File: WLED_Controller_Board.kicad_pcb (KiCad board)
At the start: 2 copper layers, 58.2 x 43.4 mm, 21 parts, among them IC1 SN74HCT125D, J1 Barrel_Jack, J2 FTDI Programmer, J3 WLED (VCC, DI, CI, GND), J4 DHT11 / DHT22, SW1 Reset, SW2 Prog, U1 ESP-12E, U2 AMS1117-3.3

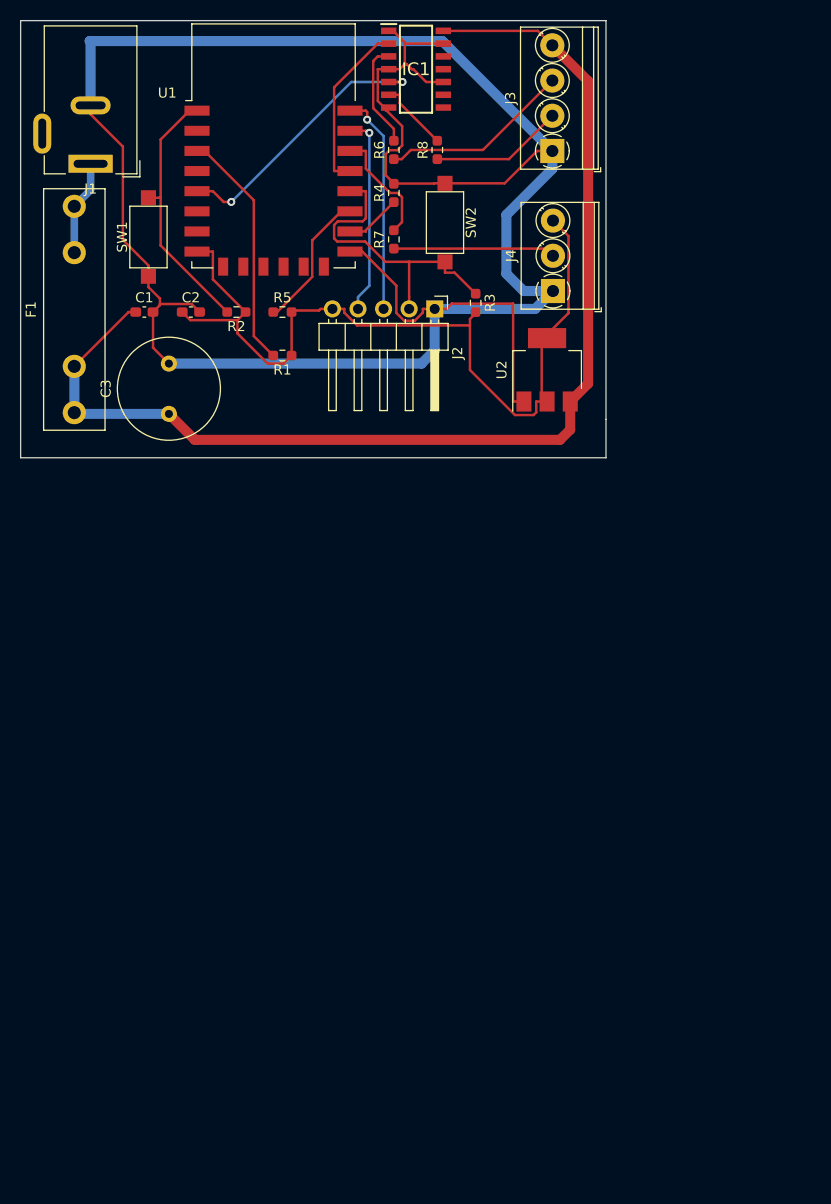
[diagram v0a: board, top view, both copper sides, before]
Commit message: Add files via upload
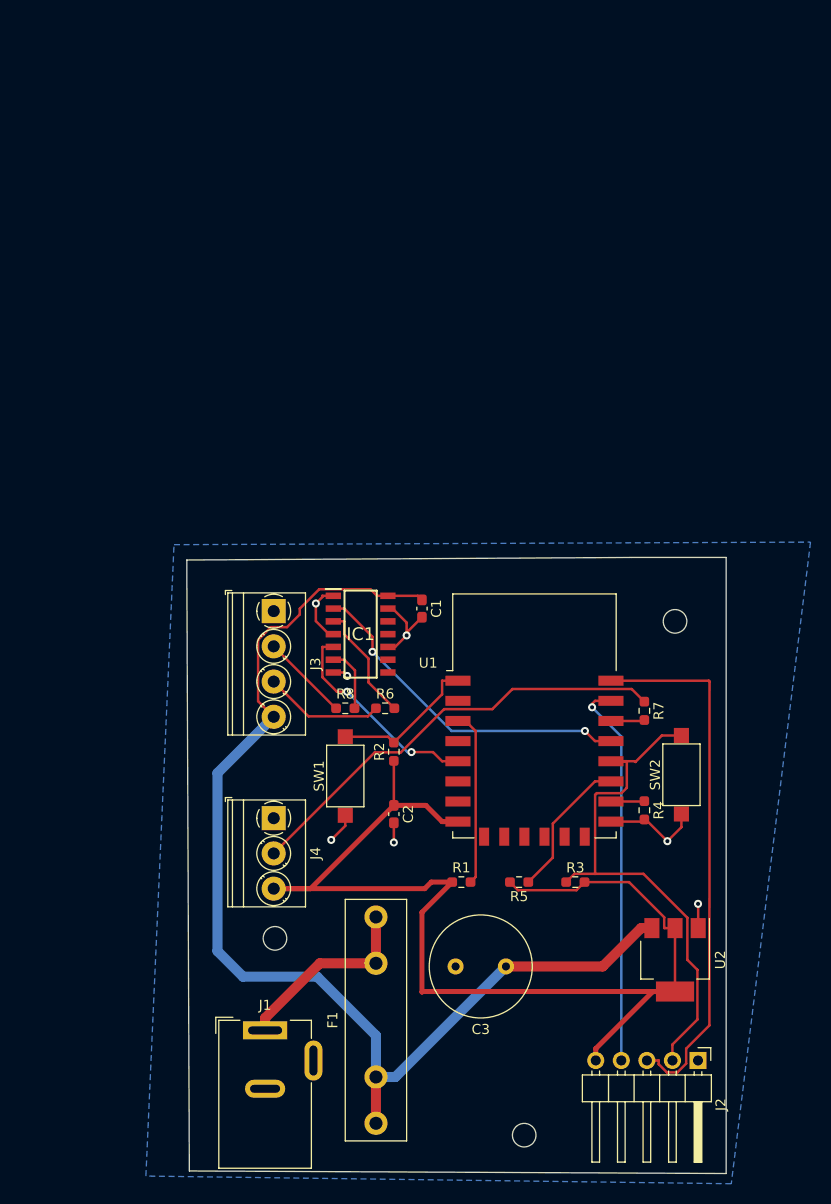
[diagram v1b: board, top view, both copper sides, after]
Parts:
- moved J1 87.8 mm to (71.3, 143.3), turned to 0 degrees
- moved J2 79.1 mm to (114.3, 146.2)
- moved F1 76.7 mm to (82.3, 152.5)
- moved R4 66.2 mm to (109.0, 121.4), turned to -90 degrees
- moved C3 64.3 mm to (95.2, 136.9), turned to 180 degrees
- moved U1 62.3 mm to (98.0, 112.0)
- moved R5 61.3 mm to (96.5, 128.5), turned to 180 degrees
- moved U2 60.0 mm to (112.0, 136.2), turned to -90 degrees
- moved SW2 59.7 mm to (112.6, 117.9), turned to 90 degrees
- moved J4 59.3 mm to (72.1, 122.2), turned to -90 degrees
- moved R3 58.4 mm to (102.1, 128.5), turned to 0 degrees
- moved SW1 57.0 mm to (79.2, 118.0)
- moved IC1 56.4 mm to (80.8, 103.9)
- moved R8 56.2 mm to (79.2, 111.3), turned to 0 degrees
- moved R6 55.5 mm to (83.2, 111.3), turned to 0 degrees
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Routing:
- net GND: track 234.2 -> 32.8 mm, vias 0 -> 7
- net +3V3: track 84.6 -> 119.8 mm
- net TX: track 22.0 -> 53.7 mm, vias 1 -> 0
- net Net-(J4-Pad2): track 16.1 -> 44.1 mm
- net GPIO0: track 30.7 -> 53.4 mm
- net RX: track 20.0 -> 38.6 mm
- net GPIO4: track 17.1 -> 33.9 mm, vias 0 -> 2
- net Net-(R2-Pad2): track 25.9 -> 14.8 mm
- net Net-(F1-Pad2): track 9.50 -> 19.1 mm
- net DHT: track 11.7 -> 3.36 mm
- net Net-(J3-Pad3): track 19.0 -> 11.9 mm
- net Net-(R1-Pad2): track 23.9 -> 17.4 mm
- net GPIO14: track 27.2 -> 21.0 mm
- net Net-(J3-Pad2): track 13.2 -> 8.75 mm
- net Net-(R4-Pad1): track 5.64 -> 3.34 mm
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- added copper zone on B.Cu, net GND
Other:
- board size 58.2 x 43.4 mm -> 53.6 x 61.2 mm
- board text added: "GND,GPIO0,TX,RX,GND"
- board text added: "VCC, DATA, Clock, GND"
- board text added: "VCC, DATA, GND"
